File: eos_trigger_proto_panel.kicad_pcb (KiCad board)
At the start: 2 copper layers, 70.5 x 37.8 mm, 70 parts, among them J1 Conn_01x02, J2 Conn_01x02, J3 Conn_01x03, J4 Conn_01x02, U2 AD8099, U3 LTC6752-1, U4 SMA-Mylibrary, U5 SMA-Mylibrary

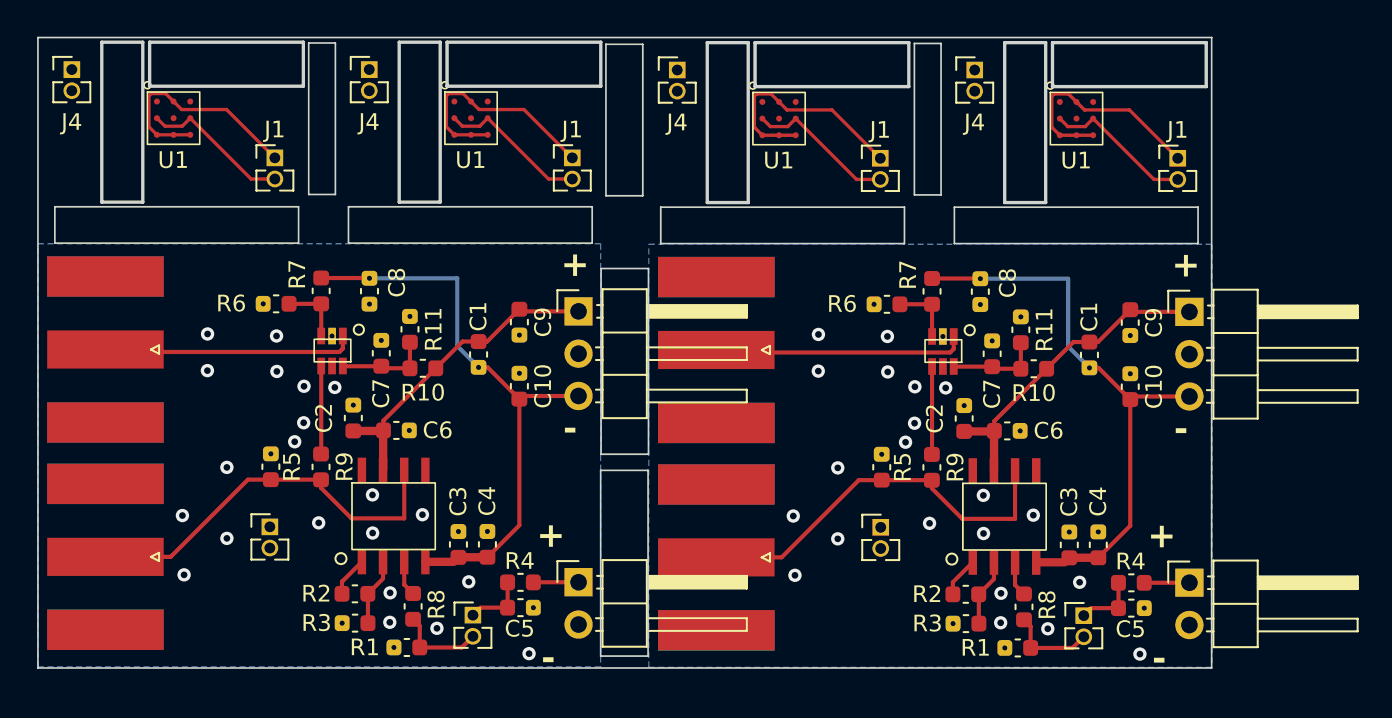
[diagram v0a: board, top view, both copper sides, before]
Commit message: tweaks
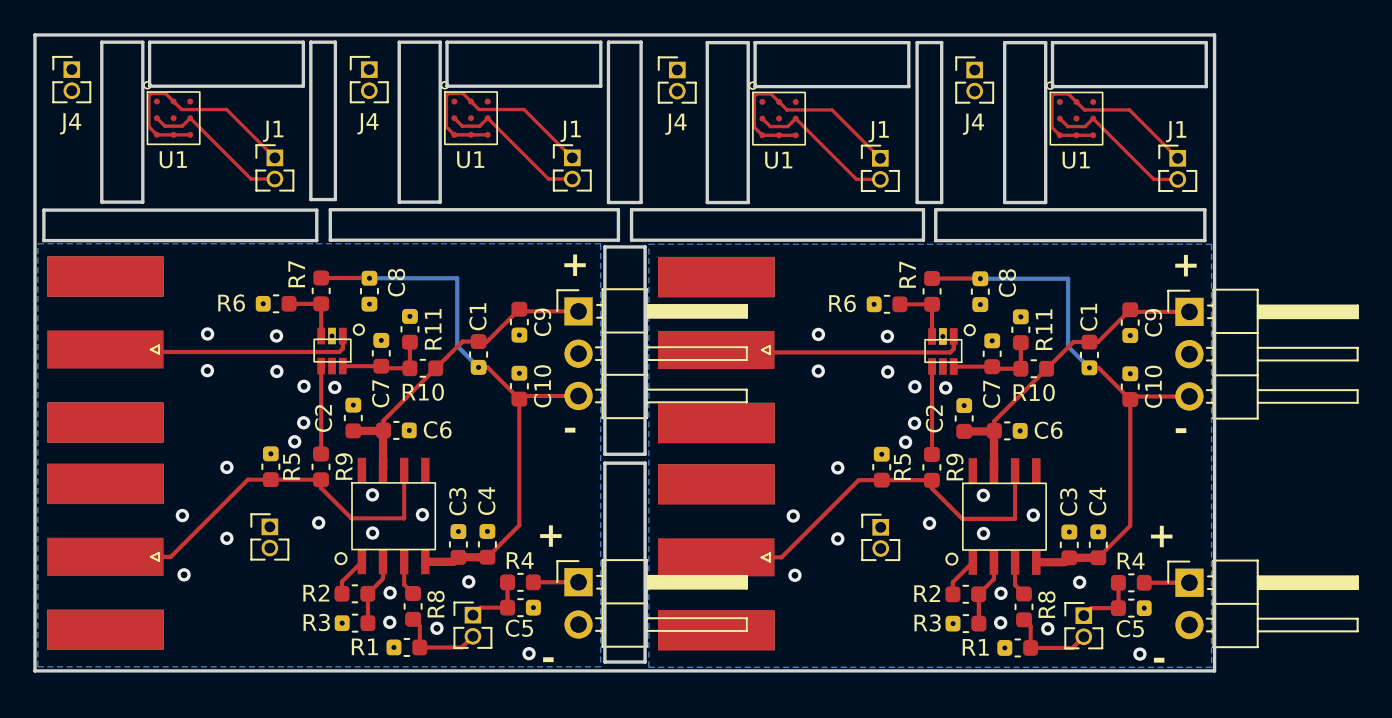
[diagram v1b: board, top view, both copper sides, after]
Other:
- board size 70.5 x 37.8 mm -> 70.8 x 38.2 mm
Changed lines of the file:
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@@
   (gr_rect (start 182.1418 70.2336) (end 191.3718 72.8736)
     (stroke (width 0.2) (type default)) (fill none) (layer "Edge.Cuts"))
-  (gr_rect (start 191.7065 70.2818) (end 193.3067 79.375)
-    (stroke (width 0.1) (type default)) (fill none) (layer "Edge.Cuts"))
-  (gr_rect (start 172.8724 95.9104) (end 175.7172 107.061)
-    (stroke (width 0.1) (type default)) (fill none) (layer "Edge.Cuts"))
   (gr_rect (start 199.998 70.2336) (end 209.228 72.8736)
     (stroke (width 0.2) (type default)) (fill none) (layer "Edge.Cuts"))
   (gr_rect (start 160.7806 70.2082) (end 163.2406 79.8082)
     (stroke (width 0.2) (type default)) (fill none) (layer "Edge.Cuts"))
-  (gr_rect (start 140.1064 80.0862) (end 154.7368 82.2706)
-    (stroke (width 0.1) (type default)) (fill none) (layer "Edge.Cuts"))
-  (gr_rect (start 155.3464 70.2564) (end 156.9466 79.3496)
-    (stroke (width 0.1) (type default)) (fill none) (layer "Edge.Cuts"))
+  (gr_rect (start 139.446 80.2894) (end 155.829 82.1182)
+    (stroke (width 0.2) (type default)) (fill none) (layer "Edge.Cuts"))
+  (gr_rect (start 191.8716 70.231) (end 193.3448 79.8322)
+    (stroke (width 0.2) (type default)) (fill none) (layer "Edge.Cuts"))
+  (gr_rect (start 155.4734 70.2056) (end 156.9466 79.6544)
+    (stroke (width 0.2) (type default)) (fill none) (layer "Edge.Cuts"))
   (gr_rect (start 163.6506 70.2082) (end 172.8806 72.8482)
     (stroke (width 0.2) (type default)) (fill none) (layer "Edge.Cuts"))
-  (gr_rect (start 176.4792 80.1116) (end 191.1096 82.296)
-    (stroke (width 0.1) (type default)) (fill none) (layer "Edge.Cuts"))
-  (gr_rect (start 139.0904 69.9262) (end 209.5536 107.776)
-    (stroke (width 0.1) (type default)) (fill none) (layer "Edge.Cuts"))
-  (gr_rect (start 172.8978 83.7946) (end 175.7426 94.9452)
-    (stroke (width 0.1) (type default)) (fill none) (layer "Edge.Cuts"))
+  (gr_rect (start 138.9126 69.7738) (end 209.7278 107.95)
+    (stroke (width 0.2) (type default)) (fill none) (layer "Edge.Cuts"))
+  (gr_rect (start 174.7266 80.264) (end 192.2526 82.0928)
+    (stroke (width 0.2) (type default)) (fill none) (layer "Edge.Cuts"))
+  (gr_rect (start 192.9892 80.264) (end 209.1436 82.1182)
+    (stroke (width 0.2) (type default)) (fill none) (layer "Edge.Cuts"))
+  (gr_rect (start 173.1264 82.4992) (end 175.5394 94.9452)
+    (stroke (width 0.2) (type default)) (fill none) (layer "Edge.Cuts"))
   (gr_rect (start 145.7944 70.2082) (end 155.0244 72.8482)
     (stroke (width 0.2) (type default)) (fill none) (layer "Edge.Cuts"))
-  (gr_rect (start 157.734 80.0862) (end 172.3644 82.2706)
-    (stroke (width 0.1) (type default)) (fill none) (layer "Edge.Cuts"))
-  (gr_rect (start 173.1899 70.3326) (end 175.3997 79.4258)
-    (stroke (width 0.1) (type default)) (fill none) (layer "Edge.Cuts"))
-  (gr_rect (start 194.1068 80.1116) (end 208.7372 82.296)
-    (stroke (width 0.1) (type default)) (fill none) (layer "Edge.Cuts"))
+  (gr_rect (start 173.3423 70.2056) (end 175.2981 79.8322)
+    (stroke (width 0.2) (type default)) (fill none) (layer "Edge.Cuts"))
+  (gr_rect (start 156.6418 80.264) (end 173.9392 82.0928)
+    (stroke (width 0.2) (type default)) (fill none) (layer "Edge.Cuts"))
   (gr_rect (start 142.9244 70.2082) (end 145.3844 79.8082)
     (stroke (width 0.2) (type default)) (fill none) (layer "Edge.Cuts"))
+  (gr_rect (start 173.1264 95.4786) (end 175.5394 107.4166)
+    (stroke (width 0.2) (type default)) (fill none) (layer "Edge.Cuts"))
   (gr_rect (start 179.2718 70.2336) (end 181.7318 79.8336)
